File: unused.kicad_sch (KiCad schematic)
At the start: 1 part, among them U8 T8Q144xx

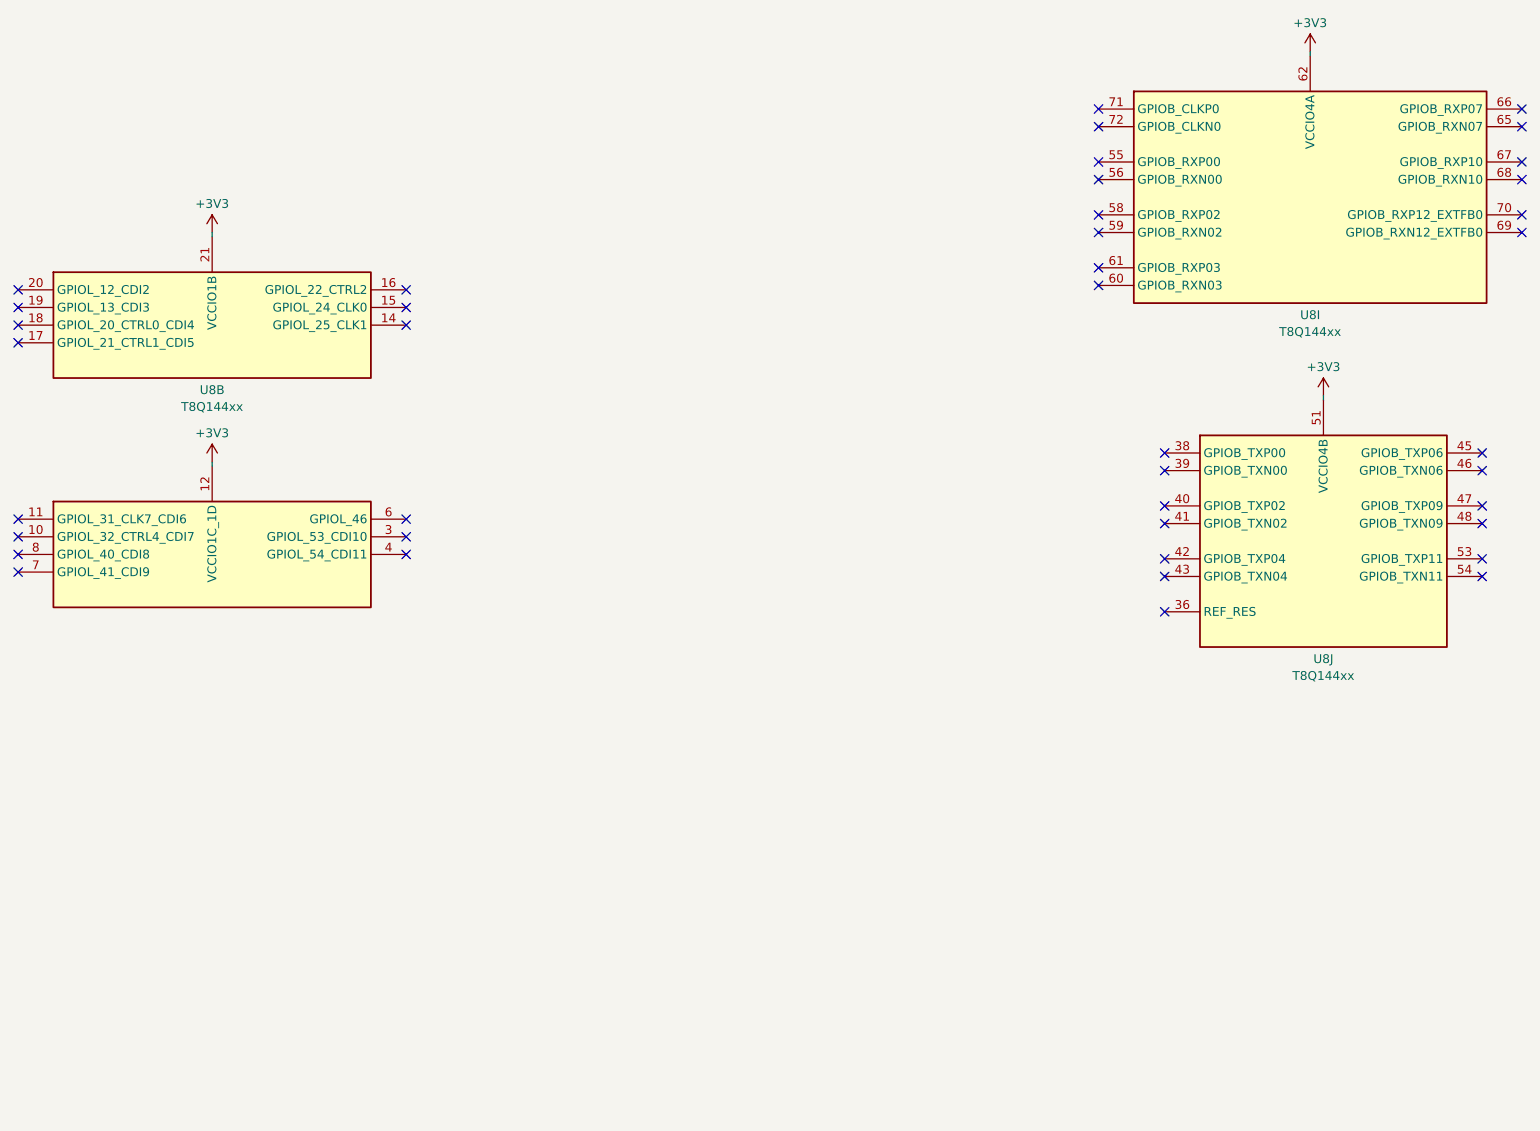
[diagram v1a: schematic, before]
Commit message: sdram layout done - COMPLETE REWORK NEEDED
cannot mix LVDS and GPIO banks due to too different timing
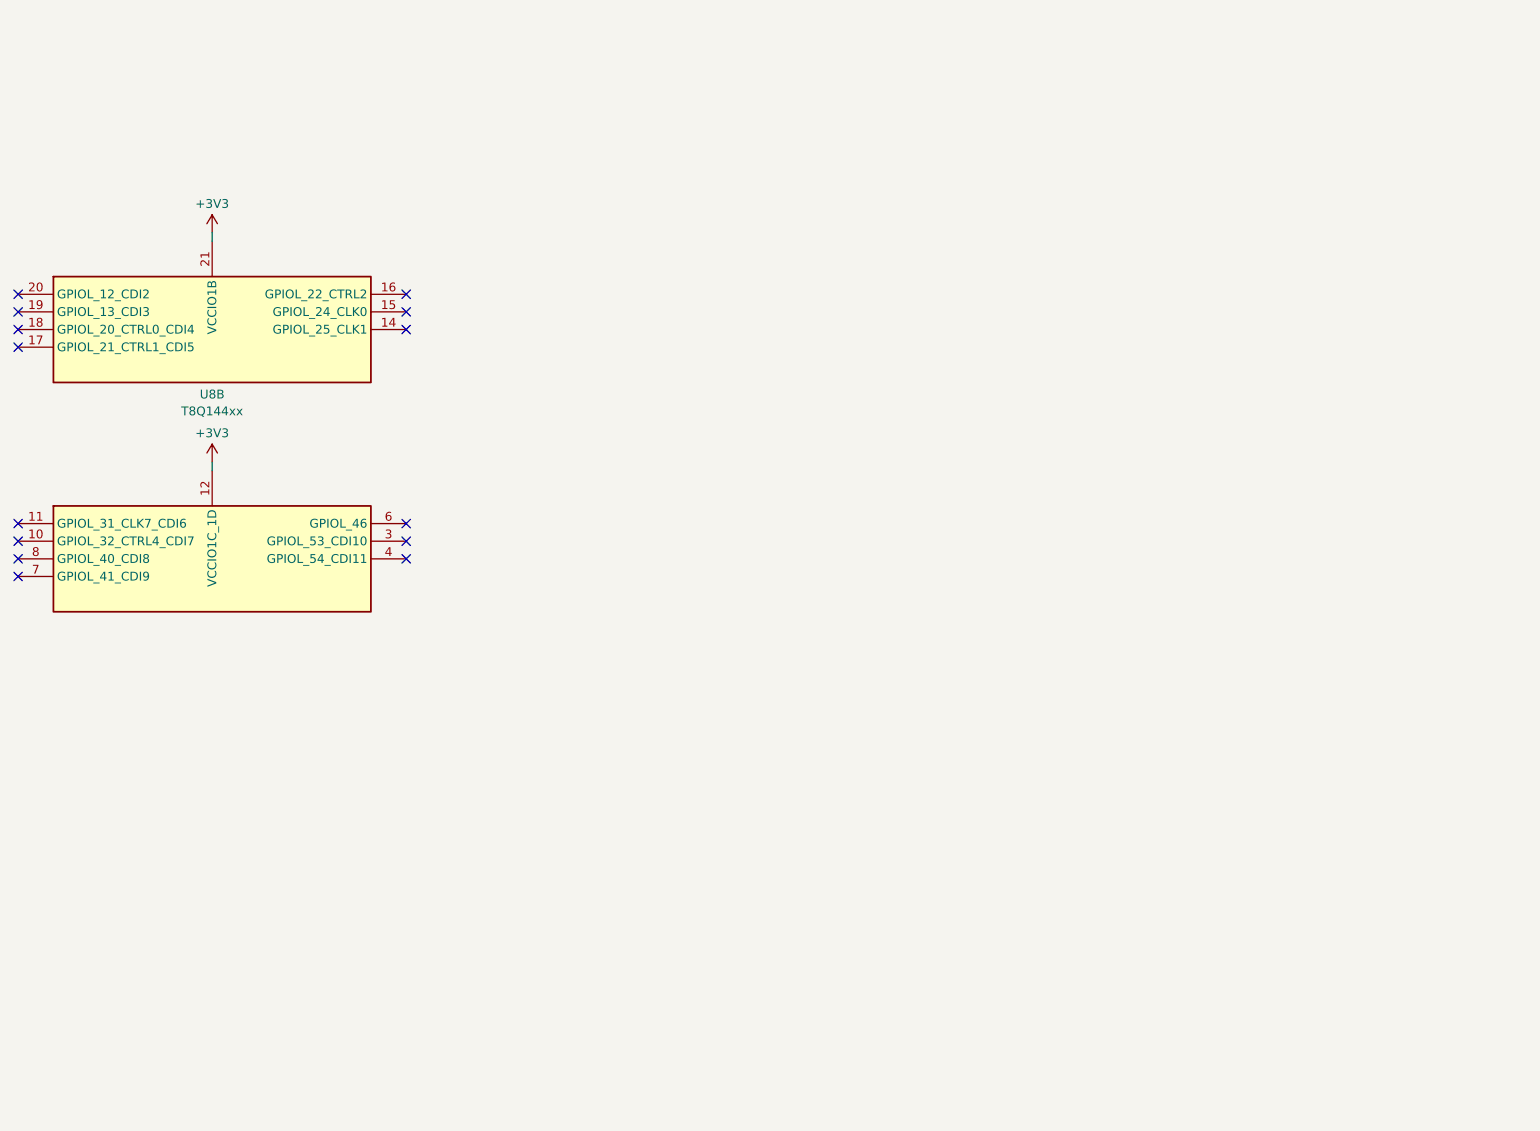
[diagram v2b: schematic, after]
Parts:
- removed unit 9 of U8
- removed unit 10 of U8
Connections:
- no-connect marks 41 -> 14
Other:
- moved on the sheet: U8B

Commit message: layout finished; passed all checks...
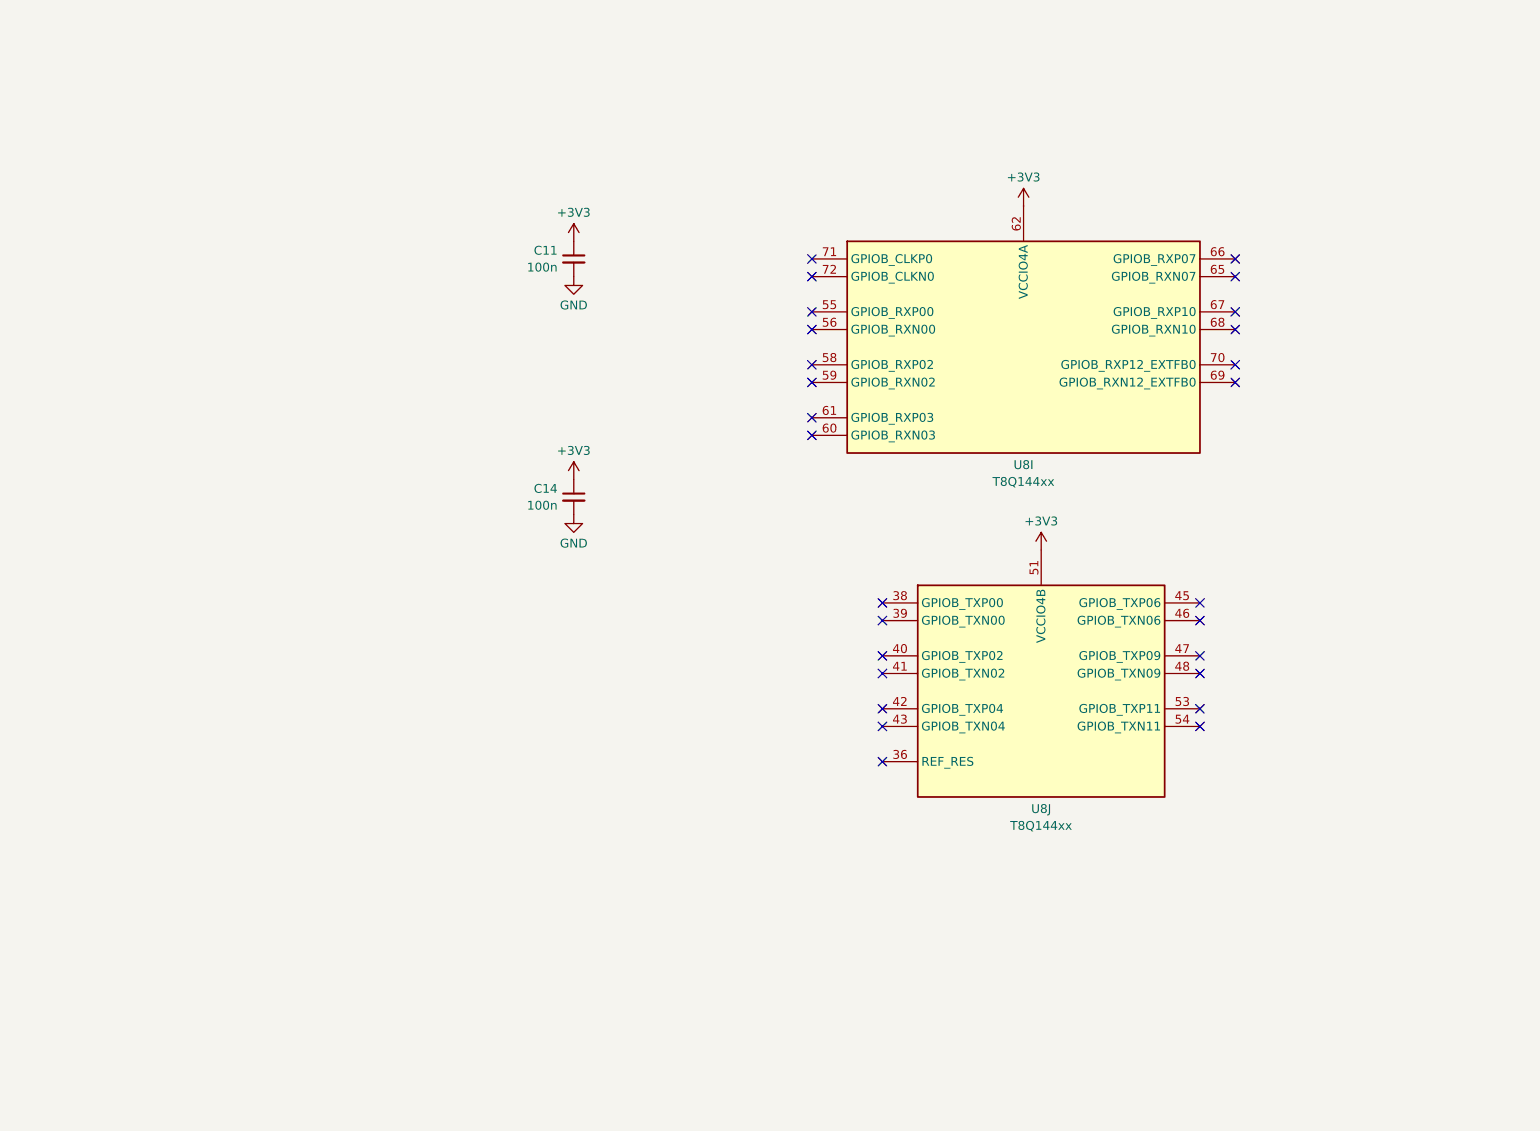
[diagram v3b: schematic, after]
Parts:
- removed U8: T8Q144xx, Package_QFP:LQFP-144_20x20mm_P0.5mm, symbol FPGA_Efinix_Trion:T8Q144xx
- added C11, C14: 100n, Capacitor_SMD:C_0603_1608Metric, symbol Device:C_Small
- added U8: T8Q144xx, Package_QFP:LQFP-144_20x20mm_P0.5mm, symbol FPGA_Efinix_Trion:T8Q144xx
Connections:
- net +3V3: now also C11.1, C14.1, U8.51 (VCCIO4B), U8.52 (VCCIO4B), U8.62 (VCCIO4A), U8.63 (VCCIO4A)
- new net GND: C11.2, C14.2
- no-connect marks 14 -> 27

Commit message: added ethernet phy
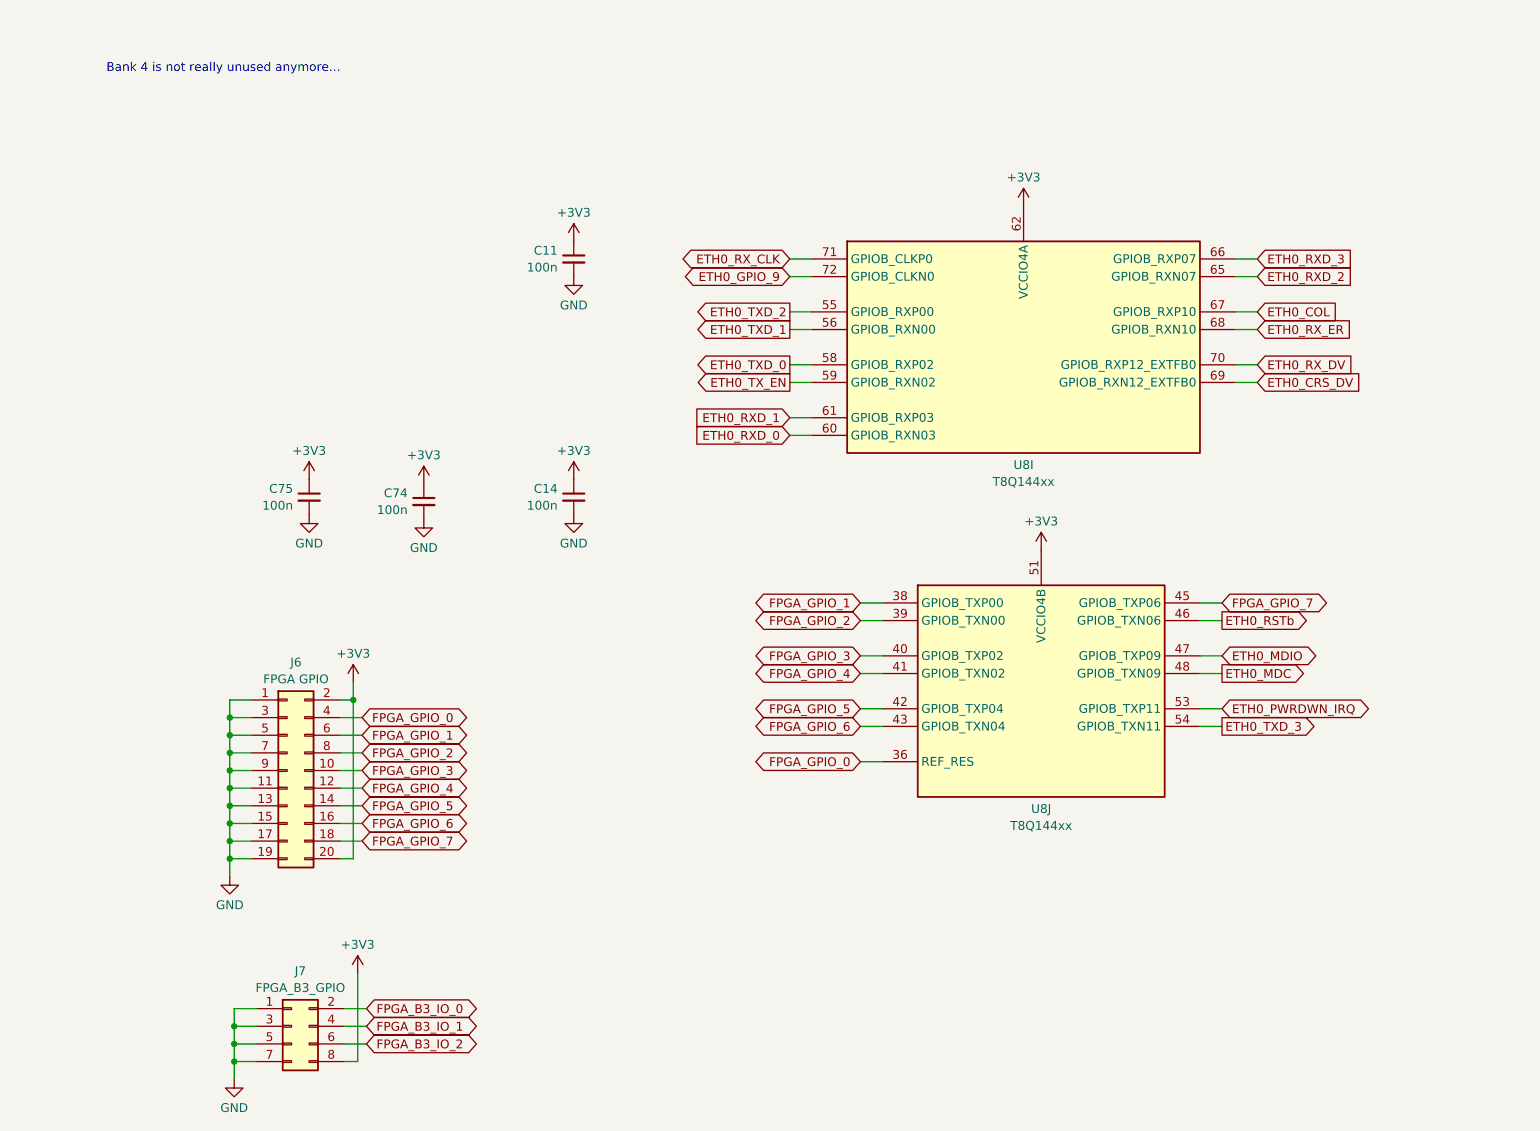
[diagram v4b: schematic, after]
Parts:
- added C74, C75: 100n, Capacitor_SMD:C_0603_1608Metric, symbol Device:C_Small
- added J6: FPGA GPIO, Connector_PinHeader_2.54mm:PinHeader_2x10_P2.54mm_Vertical, symbol Connector_Generic:Conn_02x10_Odd_Even
- added J7: FPGA_B3_GPIO, Connector_PinHeader_2.54mm:PinHeader_2x04_P2.54mm_Vertical, symbol Connector_Generic:Conn_02x04_Odd_Even
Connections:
- net +3V3: now also C74.1, C75.1, J6.2 (Pin_2), J6.20 (Pin_20), J7.8 (Pin_8)
- net GND: now also C74.2, C75.2, J6.1 (Pin_1), J6.11 (Pin_11), J6.13 (Pin_13), J6.15 (Pin_15), J6.17 (Pin_17), J6.19 (Pin_19), J6.3 (Pin_3), J6.5 (Pin_5), J6.7 (Pin_7), J6.9 (Pin_9), J7.1 (Pin_1), J7.3 (Pin_3), J7.5 (Pin_5), J7.7 (Pin_7)
- net FPGA_GPIO_0: now reaches U8.36 (REF_RES)
- net FPGA_GPIO_0: now also J6.4 (Pin_4)
- net FPGA_GPIO_1: now reaches U8.38 (GPIOB_TXP00)
- net FPGA_GPIO_1: now also J6.6 (Pin_6)
- net FPGA_GPIO_2: now reaches U8.39 (GPIOB_TXN00)
- net FPGA_GPIO_2: now also J6.8 (Pin_8)
- net FPGA_GPIO_3: now reaches U8.40 (GPIOB_TXP02)
- net FPGA_GPIO_3: now also J6.10 (Pin_10)
- net FPGA_GPIO_4: now reaches U8.41 (GPIOB_TXN02)
- net FPGA_GPIO_4: now also J6.12 (Pin_12)
- net FPGA_GPIO_5: now reaches U8.42 (GPIOB_TXP04)
- net FPGA_GPIO_5: now also J6.14 (Pin_14)
- net FPGA_GPIO_6: now reaches U8.43 (GPIOB_TXN04)
- net FPGA_GPIO_6: now also J6.16 (Pin_16)
- net FPGA_GPIO_7: now reaches U8.45 (GPIOB_TXP06)
- net FPGA_GPIO_7: now also J6.18 (Pin_18)
- net ETH0_RSTb: now reaches U8.46 (GPIOB_TXN06)
- net ETH0_MDIO: now reaches U8.47 (GPIOB_TXP09)
- net ETH0_MDC: now reaches U8.48 (GPIOB_TXN09)
- net ETH0_PWRDWN_IRQ: now reaches U8.53 (GPIOB_TXP11)
- net ETH0_TXD_3: now reaches U8.54 (GPIOB_TXN11)
- net ETH0_TXD_2: now reaches U8.55 (GPIOB_RXP00)
- net ETH0_TXD_1: now reaches U8.56 (GPIOB_RXN00)
- net ETH0_TXD_0: now reaches U8.58 (GPIOB_RXP02)
- net ETH0_TX_EN: now reaches U8.59 (GPIOB_RXN02)
- net ETH0_RXD_0: now reaches U8.60 (GPIOB_RXN03)
- net ETH0_RXD_1: now reaches U8.61 (GPIOB_RXP03)
- net ETH0_RXD_2: now reaches U8.65 (GPIOB_RXN07)
- net ETH0_RXD_3: now reaches U8.66 (GPIOB_RXP07)
- net ETH0_COL: now reaches U8.67 (GPIOB_RXP10)
- net ETH0_RX_ER: now reaches U8.68 (GPIOB_RXN10)
- net ETH0_CRS_DV: now reaches U8.69 (GPIOB_RXN12_EXTFB0)
- net ETH0_RX_DV: now reaches U8.70 (GPIOB_RXP12_EXTFB0)
- net ETH0_RX_CLK: now reaches U8.71 (GPIOB_CLKP0)
- net ETH0_GPIO_9: now reaches U8.72 (GPIOB_CLKN0)
- new net FPGA_B3_IO_0: J7.2 (Pin_2)
- new net FPGA_B3_IO_1: J7.4 (Pin_4)
- new net FPGA_B3_IO_2: J7.6 (Pin_6)
- no-connect marks 27 -> 0
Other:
- note added: "Bank 4 is not really unused anymore..."
